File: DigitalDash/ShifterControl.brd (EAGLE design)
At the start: 100.3 x 59.5 mm, 22 parts, among them IC1 7805T, J2 DT15-4P, J3 DT15-4P, J4 AVR_SPI_PROG_3X22X3_LOCK, U1 ATMEGA328P_TQFP, U2 MCP2515, U3 MCP2551, Y1 16MHz, Y2 8MHz

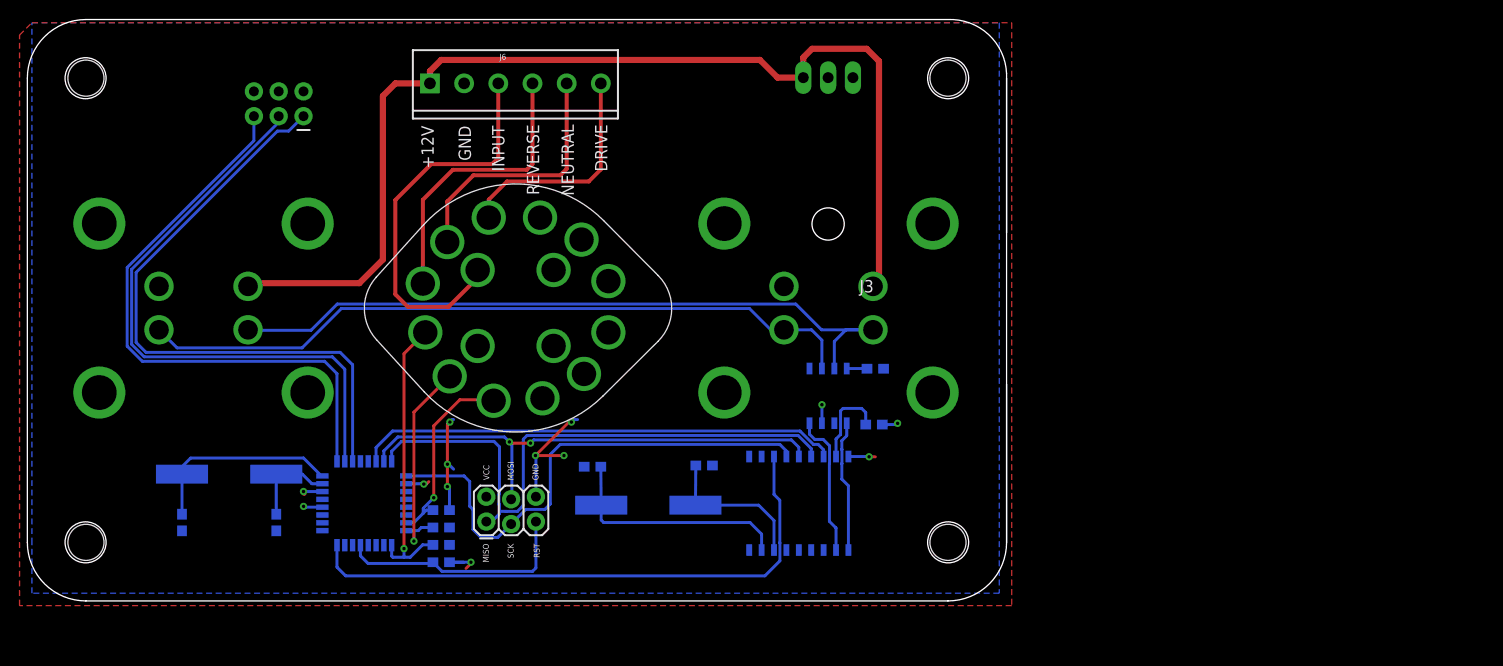
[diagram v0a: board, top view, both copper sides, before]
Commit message: add more cars
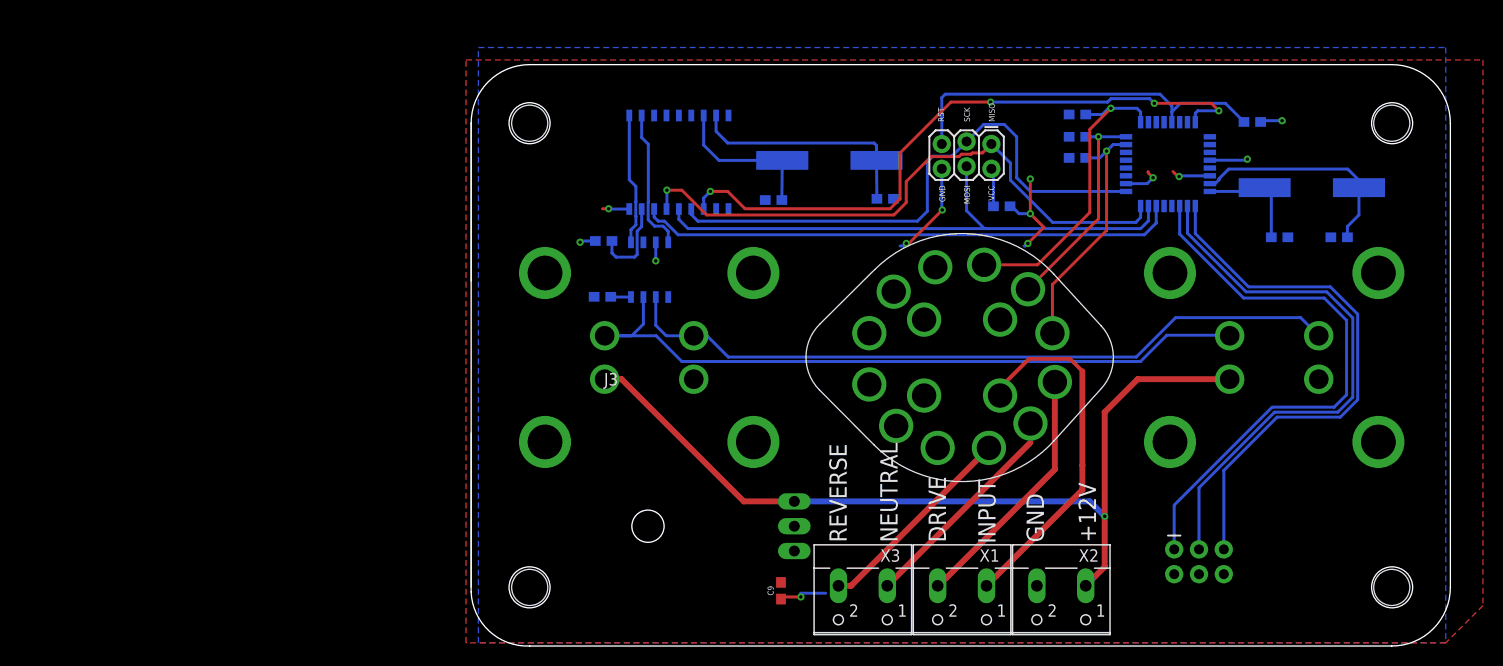
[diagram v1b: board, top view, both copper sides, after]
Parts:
- removed C3, C4: 22pF, SparkFun-Capacitors:0603
- removed J6: (no value), SparkFun-Connectors:SCREWTERMINAL-3.5MM-6
- removed R1: 1k, SparkFun-Resistors:0603
- removed U1: ATMEGA328P_TQFP, SparkFun-IC-Microcontroller:TQFP32-08
- removed Y1: 16MHz, SparkFun-Clocks:HC49UP
- added C5: 470pF, SparkFun-Capacitors:0603
- added C7, C8: 22pF, SparkFun-Capacitors:0603
- added C9: 1uF, SparkFun-Capacitors:0603
- added R7: 1k, SparkFun-Resistors:0603
- added U4: ATMEGA328P_TQFP, SparkFun-IC-Microcontroller:TQFP32-08
- added X1, X2, X3: (no value), con-wago-500:W237-102
- added Y3: 16MHz, SparkFun-Clocks:HC49UP
- moved J2 109.8 mm to (77.7, -5.08), turned to 180 degrees
- moved J1 105.3 mm to (70.0, -26.0), turned to 270 degrees
- moved R6 76.7 mm to (57.5, 19.8), turned to 180 degrees
- moved R5 76.5 mm to (57.5, 17.5), turned to 180 degrees
- moved R4 76.3 mm to (57.5, 15.4), turned to 180 degrees
- moved J4 64.7 mm to (48.7, 16.9), turned to 180 degrees
- moved U$1 46.0 mm to (45.7, -5.08), turned to 180 degrees
- moved C1 40.6 mm to (37.8, 11.2), turned to 0 degrees
- moved Y2 39.9 mm to (32.1, 15.1), turned to 180 degrees
- moved IC1 38.3 mm to (18.4, -22.3), turned to 270 degrees
- moved U2 37.0 mm to (16.7, 14.9), turned to 180 degrees
- moved R3 33.5 mm to (9.02, 6.86), turned to 180 degrees
- moved R2 28.9 mm to (8.89, 1.14), turned to 0 degrees
- moved C2 28.1 mm to (26.4, 11.0), turned to 180 degrees
- moved U3 22.4 mm to (13.7, 3.92), turned to 180 degrees
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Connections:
- removed net N$5: C4.2, U1.8, Y1.1
- removed net N$6: C3.2, U1.7, Y1.2
- new net N$10: C7.2, U4.7, Y3.2
- new net N$9: C8.2, U4.8, Y3.1
- net +12V: now also X2.1; no longer J6.1
- net CAN_INT: now also U4.32; no longer U1.32
- net CS: now also U4.14; no longer U1.14
- net DATA: now also U4.9; no longer U1.9
- net GND: now also C5.1, C7.1, C8.1, C9.1, U4.20, U4.21, U4.3, U4.5, X2.2; no longer C3.1, C4.1, J6.2, U1.20, U1.21, U1.3, U1.5
- net LATCH: now also U4.10; no longer U1.10
- net MCU_D: now also U4.23; no longer U1.25
- net MCU_N: now also U4.24; no longer U1.24
- net MCU_R: now also U4.25; no longer U1.23
- net MISO: now also U4.16; no longer U1.16
- net MOSI: now also U4.15; no longer U1.15
- net RST: now also R7.2, U4.29; no longer R1.2, U1.29
- net SCK: now also U4.17; no longer U1.17
- net SHIFT_CLK: now also U4.11; no longer U1.11
- net THROT_D: now also U$1.C2-1, X1.2; no longer J6.6, U$1.C2-3
- net THROT_INPUT: now also X1.1; no longer J6.3
- net THROT_N: now also X3.1; no longer J6.5
- net THROT_R: now also U$1.C2-3, X3.2; no longer J6.4, U$1.C2-1
- net VCC: now also C5.2, C9.2, R7.1, U4.18, U4.4, U4.6; no longer R1.1, U1.18, U1.4, U1.6
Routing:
- net N$10: track 0.00 -> 22.8 mm
- net N$5: track 20.6 -> 0.00 mm
- net +12V: track 111.8 -> 91.8 mm, vias 0 -> 1
- net RST: track 24.7 -> 39.2 mm
- net MCU_R: track 19.9 -> 31.7 mm
- net N$9: track 0.00 -> 11.1 mm
- net N$6: track 9.24 -> 0.00 mm
- net THROT_R: track 29.6 -> 21.3 mm
- net VCC: track 17.8 -> 24.5 mm
- net CAN_INT: track 59.5 -> 66.3 mm, vias 0 -> 4
- net MOSI: track 51.8 -> 58.5 mm, vias 2 -> 0
- net CS: track 49.4 -> 55.2 mm
- net SCK: track 52.0 -> 57.7 mm
- net SHIFT_CLK: track 63.9 -> 58.2 mm
- net LATCH: track 61.9 -> 57.3 mm
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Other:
- outline, holes or cut-outs redrawn
